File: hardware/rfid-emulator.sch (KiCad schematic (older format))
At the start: 95 parts, among them J1 AVR-JTAG-10, J2 Micro_USB, J3 OSTTC020162, Q1 2N3904, Q2 2N3906, Q3 2N3906, Q4 IRLML6344TRPBF, Q5 IRLML6344TRPBF, SW1 EN11-HSM1BF20, U1 NHD-C0216CiZ-FSW-FBW-3V3, U2 LT8613, U3 ATmega64A-AU, U4 MCP73832-2-OT, U5 LF33_TO252, U6 FT230XS, U7 LM324DT, Y1 ECS-160-20-5PX-TR

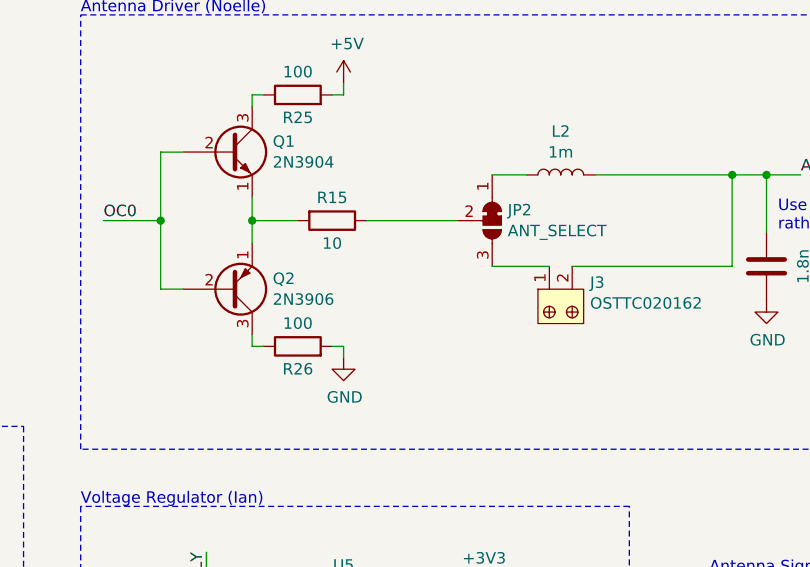
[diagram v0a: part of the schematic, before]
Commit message: Re-add Noelle's changes
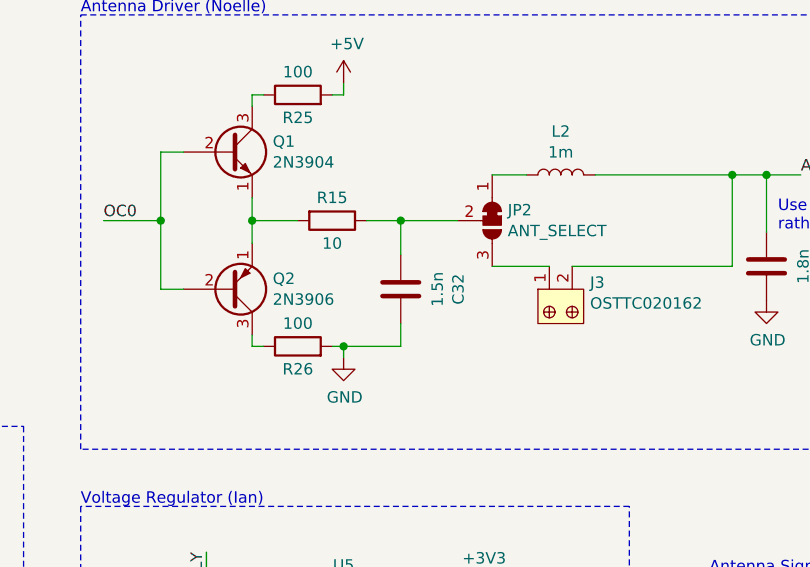
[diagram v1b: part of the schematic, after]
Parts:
- added C32: 1.5n, Capacitors_SMD:C_0805_HandSoldering, symbol Device:C
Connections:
- net GND: now also C32.1
- net at JP2.2 (C), R15.1: now also C32.2
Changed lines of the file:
@@
 $EndComp
 Wire Wire Line
-	8300 3850 8700 3850
+	8300 3850 8450 3850
 $Comp
 L Device:R R26
@@
 	13250 7350 13250 7550
 Connection ~ 13250 7550
+$Comp
+L Device:C C32
+U 1 1 5DD510A8
+P 8450 4150
+F 0 "C32" V 8198 4150 50  0000 C CNN
+F 1 "1.5n" V 8289 4150 50  0000 C CNN
+F 2 "Capacitors_SMD:C_0805_HandSoldering" H 8488 4000 50  0001 C CNN
+F 3 "~" H 8450 4150 50  0001 C CNN
+	1    8450 4150
+	-1   0    0    1
+$EndComp
+Wire Wire Line
+	8450 4300 8450 4400
+Wire Wire Line
+	8450 4400 8200 4400
+Connection ~ 8200 4400
+Wire Wire Line
+	8450 4000 8450 3850
+Connection ~ 8450 3850
+Wire Wire Line
+	8450 3850 8700 3850
 $EndSCHEMATC
